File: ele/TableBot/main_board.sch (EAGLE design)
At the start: 125 parts, among them IC1 MCP602ST, K1 ARK550/2, X4 POWER_IN

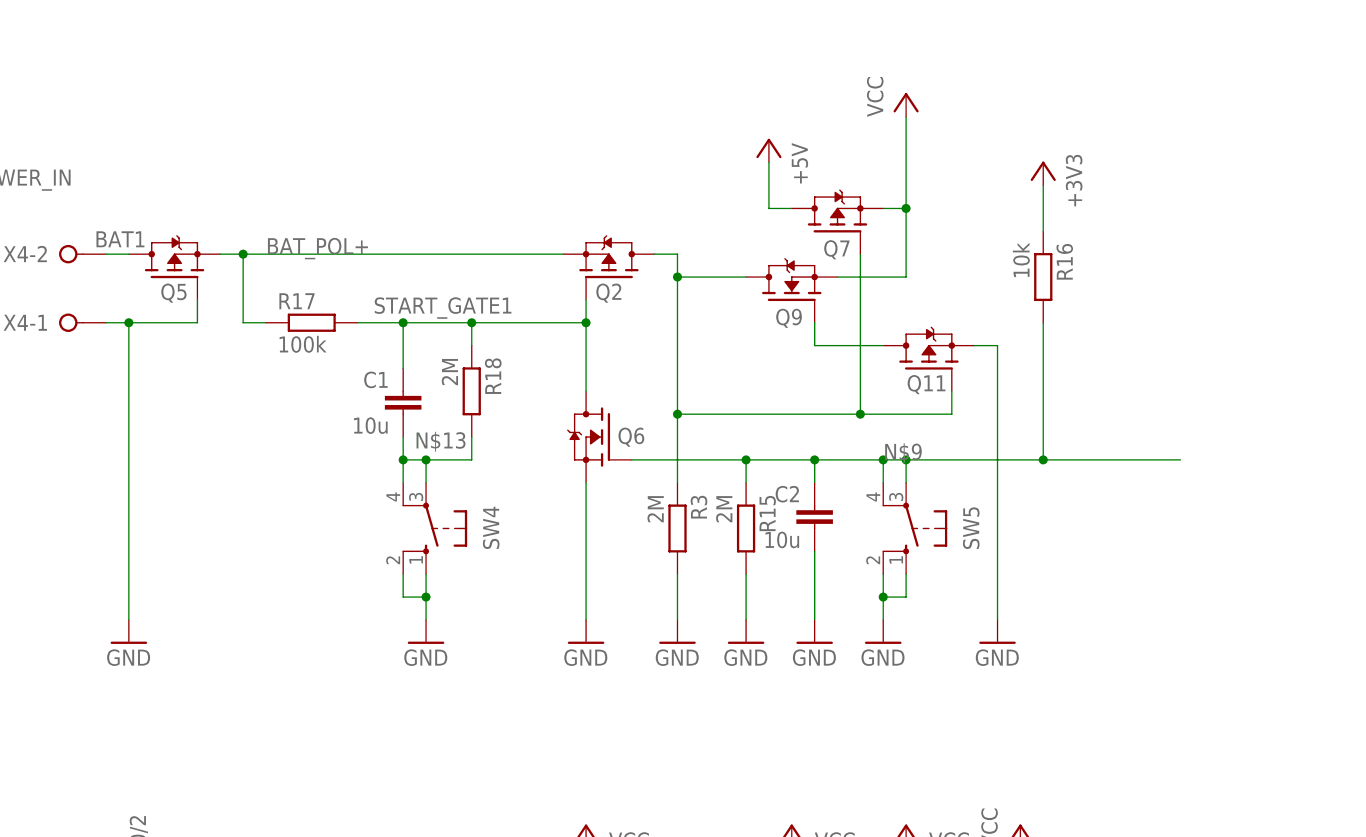
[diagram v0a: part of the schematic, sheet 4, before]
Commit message: dalsi_text_a_firstbot
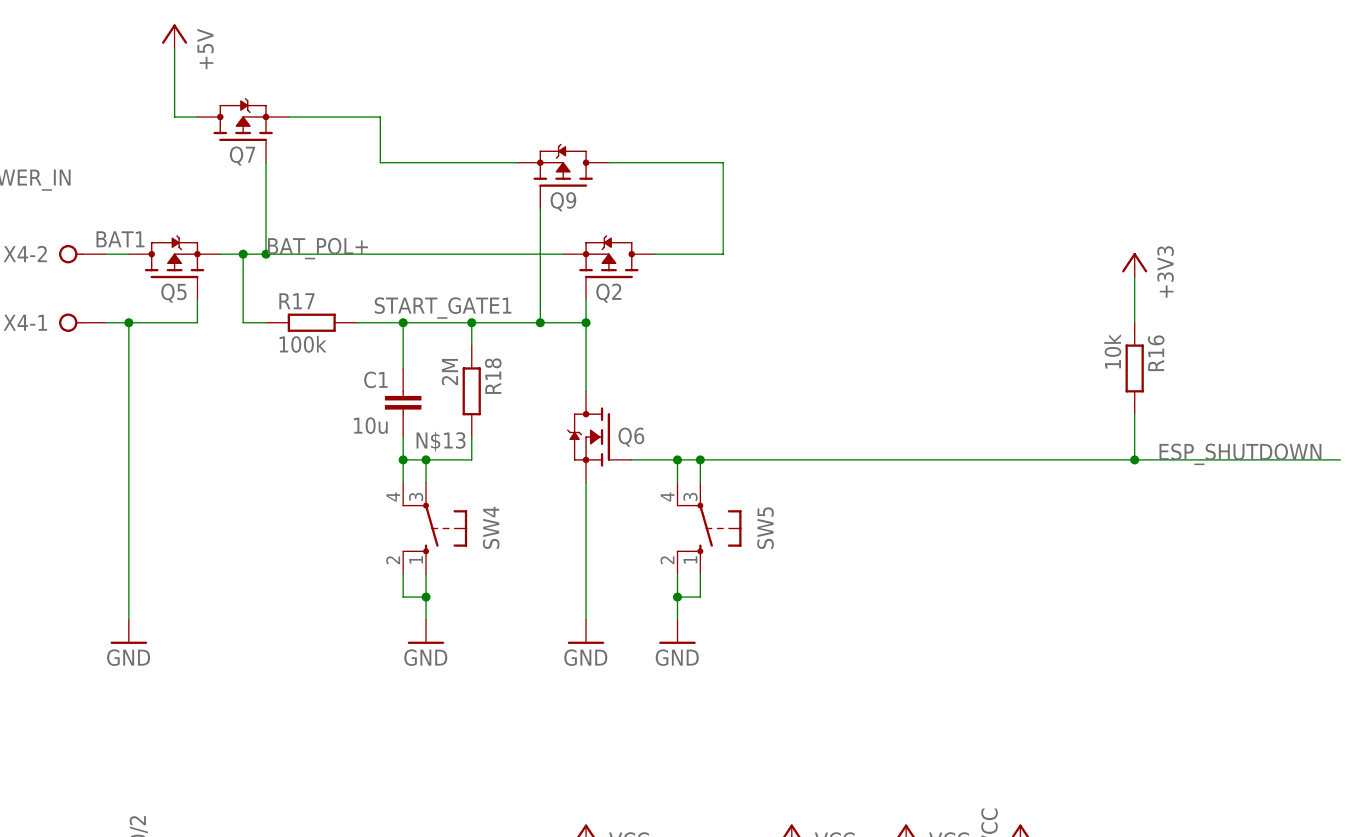
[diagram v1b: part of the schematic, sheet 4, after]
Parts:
- removed C2: 10u, rcl_upravena:C-EUC1206
- removed Q11: (no value), transistors:P-MOSFET-MLP_HS
- removed R15, R3: 2M, rcl_upravena:R-EU_R0805
- Q9: device transistors:N-MOSFET-SOT23-GSD -> transistors:P-MOSFET-MLP_HS
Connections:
- removed net N$37: Q11.D, Q9.G
- new net ESP_SHUTDOWN: Q6.G, R16.2, SW5.P, SW5.P1
- net BAT_POL+: now also Q7.G
- net GND: no longer C2.2, Q11.S, R15.2, R3.2
- net N$7: no longer Q11.G, Q7.G, R3.1
- net N$9: now also Q7.S, Q9.S; no longer C2.1, Q6.G, R15.1, R16.2, SW5.P, SW5.P1
- net START_GATE1: now also Q9.G
- net VCC: no longer Q7.S, Q9.S
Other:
- moved on the sheet: Q7, Q9, R16, SW5
